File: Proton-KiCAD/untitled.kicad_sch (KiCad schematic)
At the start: 46 parts, among them J11 FRONT_BUTTON_1, J12 FRONT_BUTTON_2, J2 KEYPAD, J3 SJ-43514, J4 SPEAKER_OUT, J5 OLED SPI, J6 ROTARY ENCODER, J7 OLED, J8 SI4703, U5 TL072, U6 LM386

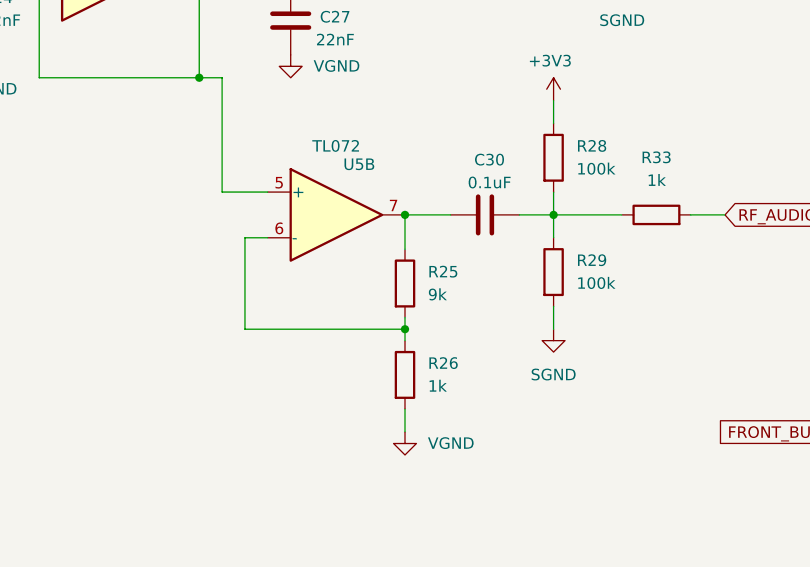
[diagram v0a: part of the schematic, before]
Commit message: saving
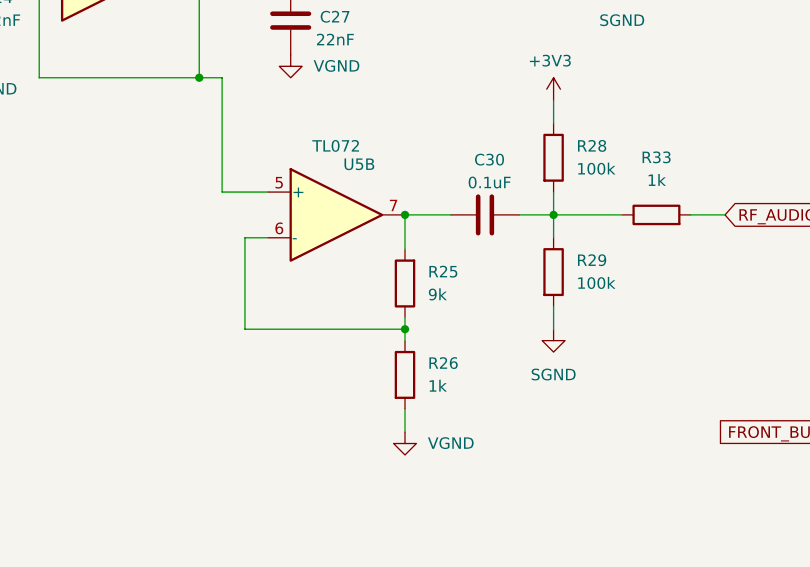
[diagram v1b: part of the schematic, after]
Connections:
- net at R26.1, U5.6 (-): now also R25.1; no longer R25.2
- net at C30.1, U5.7: now also R25.2; no longer R25.1
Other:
- moved on the sheet: R25
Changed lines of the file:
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@@
 	(symbol
 		(lib_id "Device:R")
-		(at 146.05 100.33 0)
+		(at 146.05 100.33 180)
 		(unit 1)
 		(exclude_from_sim no)
@@
 					(size 1.27 1.27)
 				)
-				(justify left)
+				(justify right)
 			)
 		)
@@
 					(size 1.27 1.27)
 				)
-				(justify left)
+				(justify right)
 			)
 		)
 		(property "Footprint" "Resistor_SMD:R_0402_1005Metric"
-			(at 144.272 100.33 90)
+			(at 147.828 100.33 90)
 			(effects
 				(font
